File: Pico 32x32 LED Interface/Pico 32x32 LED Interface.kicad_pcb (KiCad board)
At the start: 2 copper layers, 5 parts, among them J1001 Conn_01x20_Female, J1002 Conn_02x08_Odd_Even, U1001 SN74LVC4245APWR

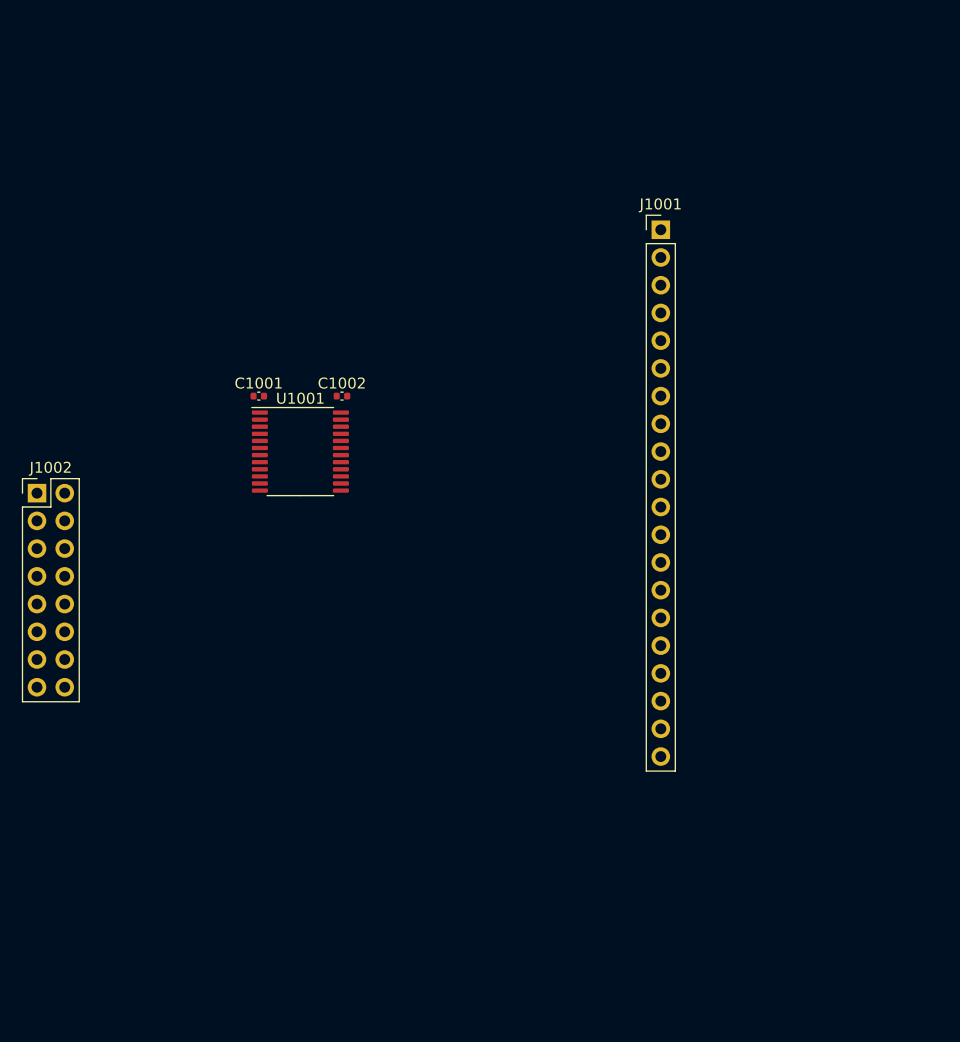
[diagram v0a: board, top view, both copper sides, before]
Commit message: Finishing draft
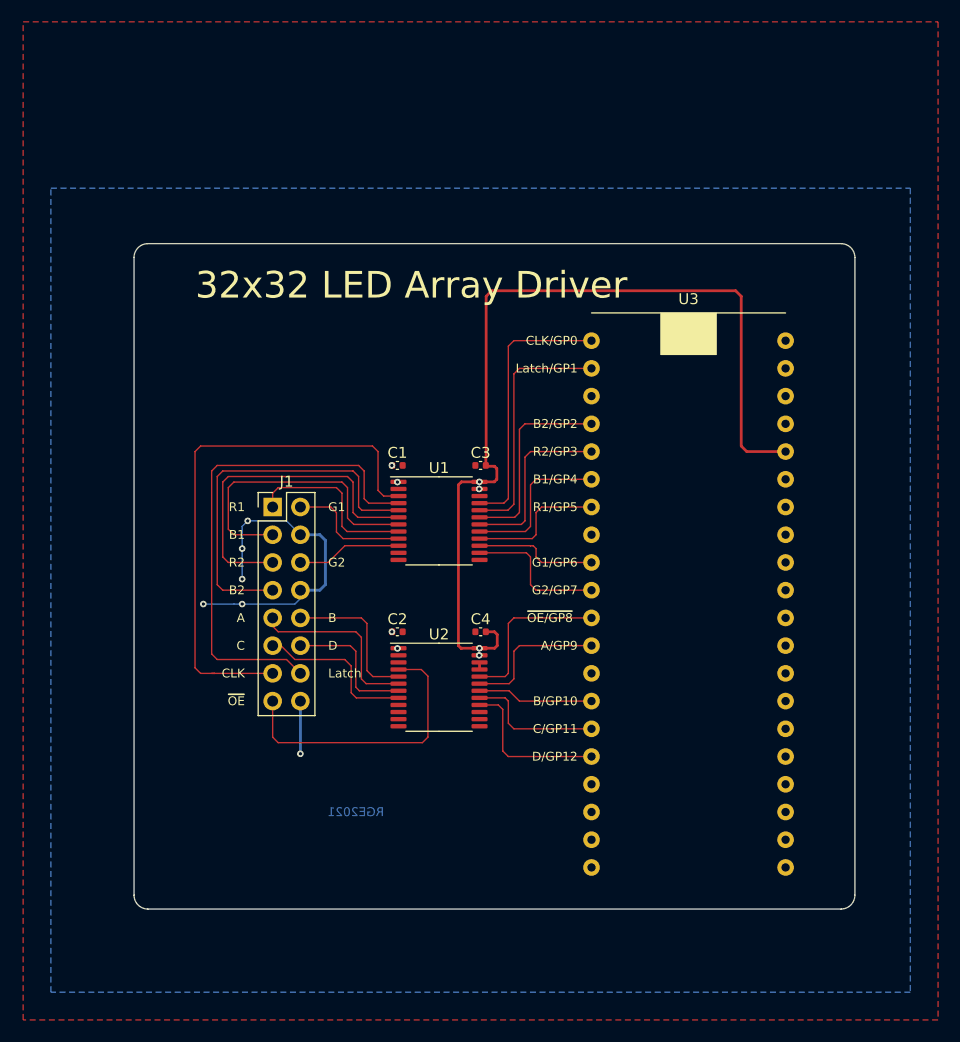
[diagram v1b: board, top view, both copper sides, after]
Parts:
- removed J1001: Conn_01x20_Female, Connector_PinHeader_2.54mm:PinHeader_1x20_P2.54mm_Vertical
- added C2: 100n, Capacitor_SMD:C_0402_1005Metric, F.Cu at (115.6, 88.9)
- added C4: 100n, Capacitor_SMD:C_0402_1005Metric, F.Cu at (123.2, 88.9)
- added U2: SN74LVC4245APWR, Package_SO:TSSOP-24_6.1x7.8mm_P0.65mm, F.Cu at (119.4, 94.0)
- added U3: Pico_Header, Pico 32x32 LED Interface:Pico_In_Headers, F.Cu at (142.2, 86.4)
- moved J1 21.6 mm to (104.1, 77.5)
- moved C3 14.2 mm to (123.2, 73.7)
- moved C1 14.2 mm to (115.6, 73.7)
- moved U1 14.2 mm to (119.4, 78.7)
- renumbered C1001 to C1, C1002 to C3, J1002 to J1, U1001 to U1
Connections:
- J1 pad 13: /CLK -> /CLKOut
- U1 pad 10: Net-(U1001-Pad10) -> /G2Out
- U1 pad 3: Net-(U1001-Pad3) -> /CLKOut
- U1 pad 4: Net-(U1001-Pad4) -> /LatchOut
- U1 pad 5: Net-(U1001-Pad5) -> /B2Out
- U1 pad 6: Net-(U1001-Pad6) -> /R2Out
- U1 pad 7: Net-(U1001-Pad7) -> /B1Out
- U1 pad 8: Net-(U1001-Pad8) -> /R1Out
- U1 pad 9: Net-(U1001-Pad9) -> /G1Out
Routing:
- net +3V3: track 0.00 -> 85.1 mm, vias 0 -> 4
- net /CLKOut: track 0.00 -> 50.2 mm
- net /LatchOut: track 0.00 -> 45.9 mm
- net GND: track 0.00 -> 35.3 mm, vias 0 -> 6
- net /B2Out: track 0.00 -> 35.1 mm
- net /R2Out: track 0.00 -> 31.1 mm
- net /B1Out: track 0.00 -> 27.1 mm
- net /~OEOut: track 0.00 -> 26.5 mm
- net Net-(U1-Pad21): track 0.00 -> 24.6 mm
- net Net-(U1-Pad20): track 0.00 -> 22.6 mm
- net Net-(U1-Pad19): track 0.00 -> 18.3 mm
- net /AOut: track 0.00 -> 16.7 mm
- net /R1Out: track 0.00 -> 16.5 mm
- net Net-(U1-Pad18): track 0.00 -> 16.4 mm
- net Net-(U2-Pad20): track 0.00 -> 15.2 mm
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- added copper zone on B.Cu, net +5V
- added copper zone on F.Cu, net GND
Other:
- board outline added: 66 x 61 mm
- board text added: "32x32 LED Array Driver"
- board text added: "A"
- board text added: "A/GP9"
- board text added: "B"
- board text added: "B/GP10"
- board text added: "B1"
- board text added: "B1/GP4"
- board text added: "B2"
- board text added: "B2/GP2"
- board text added: "C"
- board text added: "C/GP11"
- board text added: "CLK"
- board text added: "CLK/GP0"
- board text added: "D"
- board text added: "D/GP12"
- board text added: "G1"
- board text added: "G1/GP6"
- board text added: "G2"
- board text added: "G2/GP7"
- board text added: "Latch"
- board text added: "Latch/GP1"
- board text added: "R1"
- board text added: "R1/GP5"
- board text added: "R2"
- board text added: "R2/GP3"
- board text added: "RGE2021"
- board text added: "~OE"
- board text added: "~OE/GP8"
